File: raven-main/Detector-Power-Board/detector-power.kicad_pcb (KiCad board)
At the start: 2 copper layers, 37 x 52.5 mm, 38 parts, among them J1 DeployLipo, J2 Conn_01x04, J9 UCLipo, U1 LT8330IS6-TRMPBF, U2 TPS22810DRV, U3 LM317LCLPRE3, U4 LM317LCLPRE3

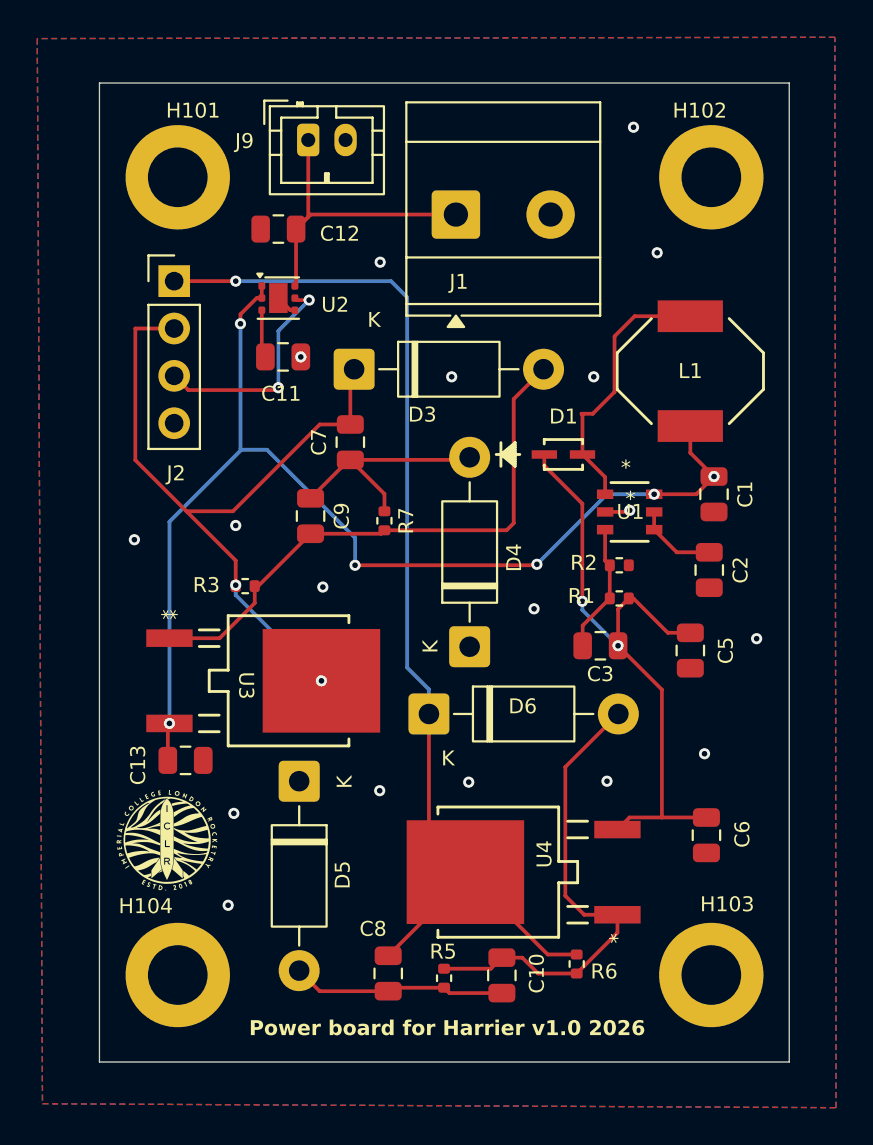
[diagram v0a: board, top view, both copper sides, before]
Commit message: power board done
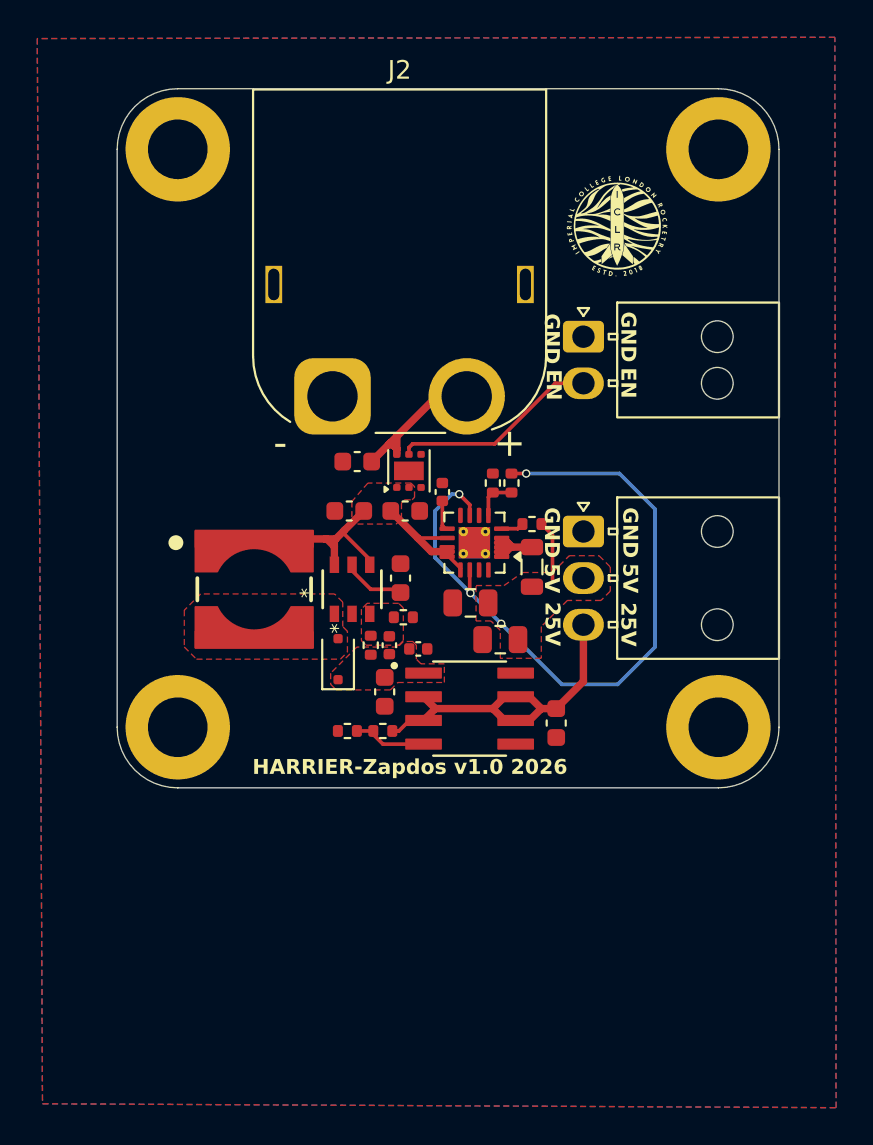
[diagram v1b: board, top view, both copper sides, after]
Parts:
- removed C12: 5u, Capacitor_SMD:C_0805_2012Metric
- removed C13: 0.1u, Capacitor_SMD:C_0805_2012Metric
- removed D3, D4, D5, D6: 1N4002, Diode_THT:D_DO-41_SOD81_P10.16mm_Horizontal
- removed the G*** at (139.3, 83.7)
- removed J9: UCLipo, Connector_JST:JST_PH_B2B-PH-K_1x02_P2.00mm_Vertical
- removed the U3 at (120.9, 89.5)
- added C4: 4.7pF 50V, Capacitor_SMD:C_0402_1005Metric, F.Cu at (126.3, 87.6)
- added G***: LOGO, LOGO, B.Cu at (127.0, 84.0)
- added J3: Conn_01x03_Pin, Connector_Molex:Molex_Nano-Fit_105313-xx03_1x03_P2.50mm_Horizontal, F.Cu at (136.8, 81.5)
- added L2: 2.2uH, Inductor_SMD:L_0805_2012Metric, F.Cu at (134.0, 83.4)
- added R4: 10k, Resistor_SMD:R_0402_1005Metric, F.Cu at (127.1, 86.1)
- added U4: TPS62150, Package_DFN_QFN:VQFN-16-1EP_3x3mm_P0.5mm_EP1.68x1.68mm_ThermalVias, F.Cu at (130.9, 82.1)
- C1: value 4.7u -> 4.7uF 50V; footprint Capacitor_SMD:C_0805_2012Metric -> Capacitor_SMD:C_0603_1608Metric
- C10, C9: value 1u -> 10uF
- C11: value 1n -> 620pF; footprint Capacitor_SMD:C_0805_2012Metric -> Capacitor_SMD:C_0402_1005Metric
- C2, C8: value 1u -> 4.7uF; footprint Capacitor_SMD:C_0805_2012Metric -> Capacitor_SMD:C_0603_1608Metric
- C3: value 4.7p -> 4.7uF 50V; footprint Capacitor_SMD:C_0805_2012Metric -> Capacitor_SMD:C_0603_1608Metric
- C5: value 4.7u -> 100nF 50V; footprint Capacitor_SMD:C_0805_2012Metric -> Capacitor_SMD:C_0402_1005Metric
- C6: value 0.1u -> 1uF 50V; footprint Capacitor_SMD:C_0805_2012Metric -> Capacitor_SMD:C_0603_1608Metric
- C7: value 1u -> 1uF; footprint Capacitor_SMD:C_0805_2012Metric -> Capacitor_SMD:C_0603_1608Metric
- D1: value D_Schottky -> PMEG6010CEJ; footprint PMEG4010BEA:SOD323F_NEX -> Diode_SMD:D_SOD-323F
- J1: value DeployLipo -> Conn_01x02_Pin; footprint TerminalBlock_Phoenix:TerminalBlock_Phoenix_MKDS-3-2-5.08_1x02_P5.08mm_Horizontal -> Connector_Molex:Molex_Nano-Fit_105313-xx02_1x02_P2.50mm_Horizontal
- J2: value Conn_01x04 -> DeployLipo; footprint Connector_PinHeader_2.54mm:PinHeader_1x04_P2.54mm_Vertical -> Connector_AMASS:AMASS_XT60PW-M_1x02_P7.20mm_Horizontal
- L1: value 8.2u -> 6.8uH; footprint CDR7D28MNNP-8R0NC:IND_8R0NC_SUM -> iclr:WE-HEPC_6030
- R2: value 10k -> 240Ω
- R3: value 240 -> 4.56kΩ
- R5: value 4.56k -> 100k
- R6: value 240 -> 953k
- R7: value 720 -> 180k
- U2: renamed from U4; value LM317LCLPRE3 -> LM317LIDR; footprint LM317MDT_TR:DPAK_STM -> iclr:SOIC127P599X175-8N
- moved G*** 40.8 mm to (138.6, 65.1)
- moved L1 26.2 mm to (119.1, 84.6), turned to 0 degrees
- moved R6 26.0 mm to (132.9, 78.9)
- moved C8 24.8 mm to (127.2, 80.4), turned to 0 degrees
- moved R5 24.8 mm to (134.0, 81.1), turned to 180 degrees
- moved C10 20.0 mm to (130.7, 85.3), turned to 180 degrees
- moved C2 19.6 mm to (124.2, 80.4), turned to 180 degrees
- moved C1 19.2 mm to (124.6, 77.8), turned to 180 degrees
- moved G*** 17.7 mm to (125.0, 67.5)
- moved D1 16.3 mm to (123.6, 88.3), turned to 90 degrees
- moved R2 15.5 mm to (126.0, 92.2), turned to 180 degrees
- moved U3 15.5 mm to (124.3, 84.6), turned to 90 degrees
- moved C5 14.6 mm to (127.9, 87.8), turned to 0 degrees
- moved R1 13.6 mm to (125.3, 87.6), turned to 90 degrees
- moved H3 13.3 mm to (144.0, 92.0)
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- renumbered H101 to H1, H102 to H2, H103 to H3, H104 to H4, U2 to U1, U1 to U3
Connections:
- C1 pad 1: /BBIN -> /BATT+
- C10 pad 1: Net-(D5-A) -> /Power_Out_5V
- C10 pad 2: Net-(D6-A) -> GND
- C11 pad 1: Net-(U2-CT) -> Net-(U4-SS/TR)
- C2 pad 1: Net-(U1-EN/UVLO) -> /BBIN
- C3 pad 2: Net-(U1-FBX) -> GND
- C6 pad 1: /Power_Out_27.5V -> /Filtered_Power_Out_25V
- C7 pad 1: Net-(D4-A) -> Net-(U3-INTVCC)
- C7 pad 2: /Power_Out_5V -> GND
- C8 pad 1: Net-(D5-A) -> /BBIN
- C8 pad 2: /Filtered_Power_Out_25V -> GND
- C9 pad 1: Net-(D4-A) -> /Power_Out_5V
- C9 pad 2: Net-(D3-A) -> GND
- J1 pad 1: Net-(J1-Pin_1) -> GND
- J1 pad 2: GND -> /ON-OFF
- J2 pad 1: /Filtered_Power_Out_25V -> GND
- J2 pad 2: /Power_Out_5V -> /BATT+
- R1 pad 2: Net-(U1-FBX) -> Net-(U3-FBX)
- R2 pad 1: Net-(U1-FBX) -> /Filtered_Power_Out_25V
- R2 pad 2: GND -> Net-(U2-ADJUST)
- R3 pad 1: Net-(D3-A) -> Net-(U2-ADJUST)
- R3 pad 2: /Power_Out_5V -> GND
- R5 pad 1: Net-(D6-A) -> /Power_Out_5V
- R5 pad 2: Net-(D5-A) -> Net-(U4-PG)
- R6 pad 1: /Filtered_Power_Out_25V -> /Power_Out_5V
- R6 pad 2: Net-(D6-A) -> Net-(U4-FB)
- R7 pad 1: Net-(D4-A) -> Net-(U4-FB)
- R7 pad 2: Net-(D3-A) -> GND
- U1 pad 3: Net-(U2-CT) -> unconnected-(U1-CT-Pad3)
- U1 pad 4: Net-(U2-GND-Pad4) -> GND
- U1 pad 6: Net-(J1-Pin_1) -> /BATT+
- U1 pad 7: Net-(U2-GND-Pad4) -> GND
- U2 pad 1: Net-(D6-A) -> /Power_Out_27.5V
- U2 pad 2: /Power_Out_27.5V -> /Filtered_Power_Out_25V
- U3 pad 3: Net-(U1-FBX) -> Net-(U3-FBX)
- U3 pad 4: Net-(U1-EN/UVLO) -> /BBIN
- U3 pad 5: Net-(U1-EN/UVLO) -> Net-(U3-INTVCC)
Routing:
- net /BBIN: track 61.9 -> 17.8 mm, vias 6 -> 0
- net /Filtered_Power_Out_25V: track 60.6 -> 18.9 mm, vias 1 -> 0
- net /Power_Out_27.5V: track 34.2 -> 0.00 mm, vias 2 -> 0
- net Net-(D3-A): track 30.5 -> 0.00 mm
- net Net-(D6-A): track 25.9 -> 0.00 mm
- net Net-(J1-Pin_1): track 17.0 -> 0.00 mm
- net Net-(D1-A): track 14.6 -> 0.00 mm
- net Net-(D4-A): track 13.0 -> 0.00 mm
- net Net-(D5-A): track 11.5 -> 0.00 mm
- net /BATT+: track 0.00 -> 8.39 mm
- net Net-(U1-FBX): track 6.94 -> 0.00 mm
- net Net-(U1-EN/UVLO): track 4.41 -> 0.00 mm
- net Net-(U2-ADJUST): track 0.00 -> 4.16 mm
- net Net-(U3-INTVCC): track 0.00 -> 3.26 mm
- net Net-(L2-Pad1): track 0.00 -> 2.82 mm
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- added copper zone on F.Cu, net /BBIN
- added copper zone on F.Cu, net /Power_Out_27.5V
- added copper zone on F.Cu, net /Power_Out_5V
- added copper zone on F.Cu, net Net-(D1-A)
- added copper zone on F.Cu, net Net-(U3-FBX)
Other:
- board size 37 x 52.5 mm -> 35.5 x 37.5 mm
- board text added: "25V"
- board text added: "5V"
- board text added: "EN"
- board text added: "GND"
- board text added: "HARRIER-Zapdos v1.0"
- board text added: "HARRIER-Zapdos v1.0 2026"
- board text removed: "Power Board for HARRIER v1.0"
- board text removed: "Power board for Harrier v1.0 2026"
